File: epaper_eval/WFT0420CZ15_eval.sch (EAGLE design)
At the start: 15 parts, among them CN1 WFT0420CZ15_IF, CN2 WFT0420CZ15

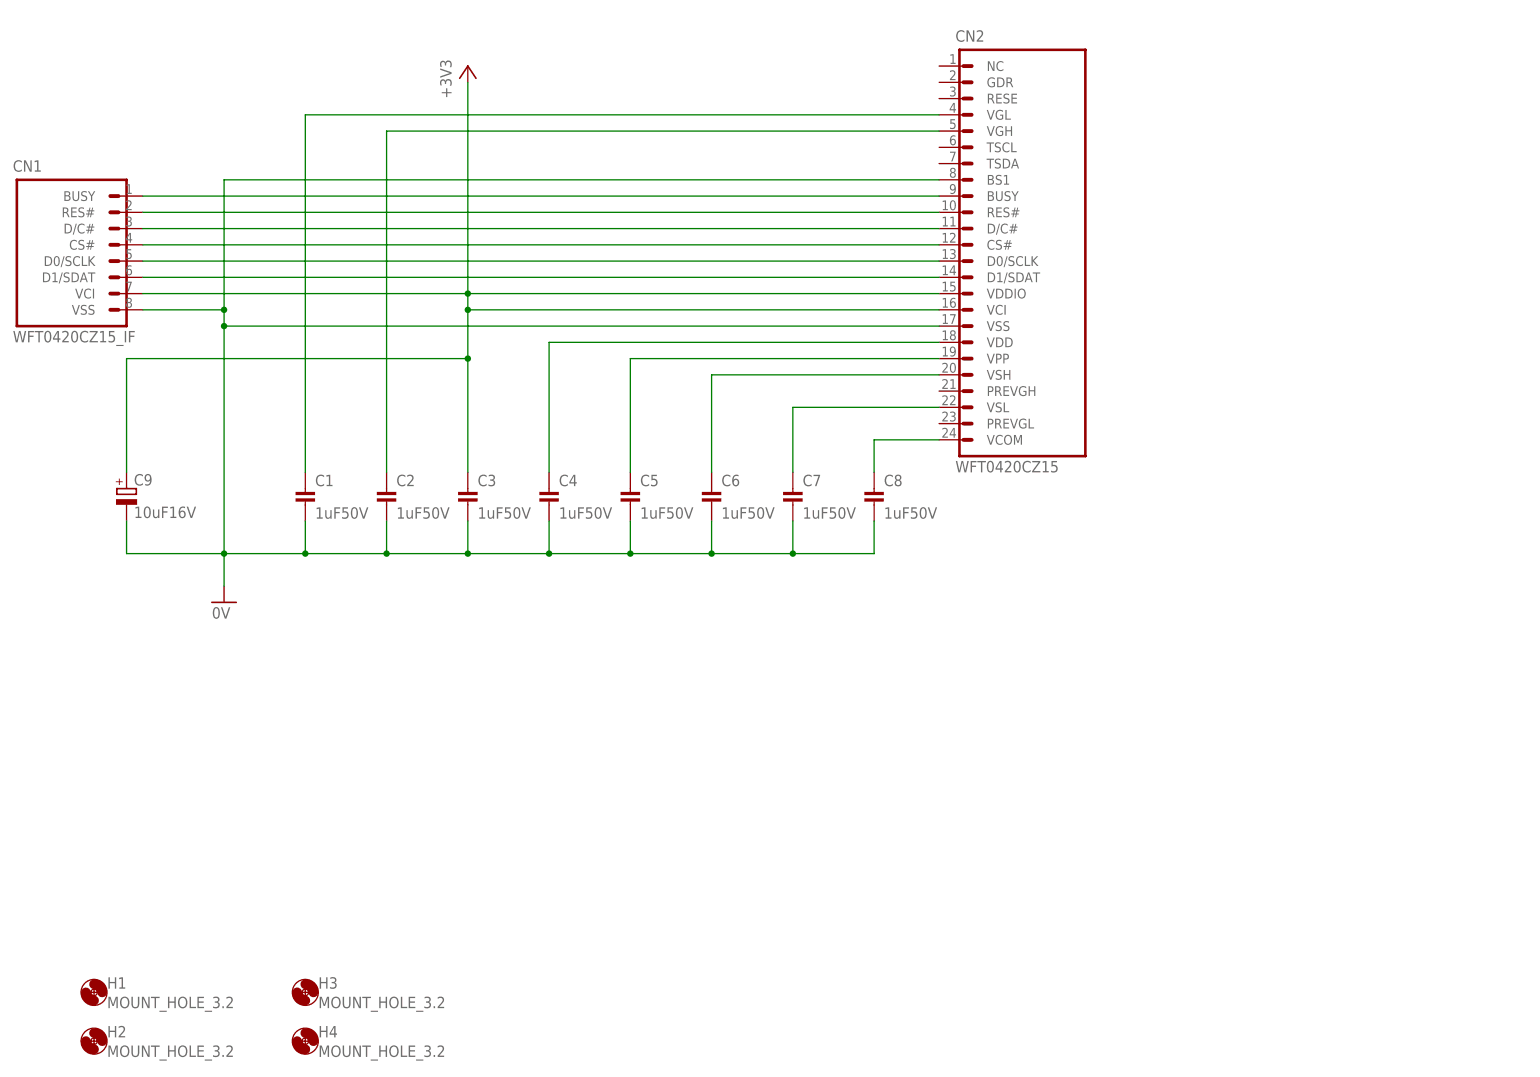
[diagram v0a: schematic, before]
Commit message: 部品を追加
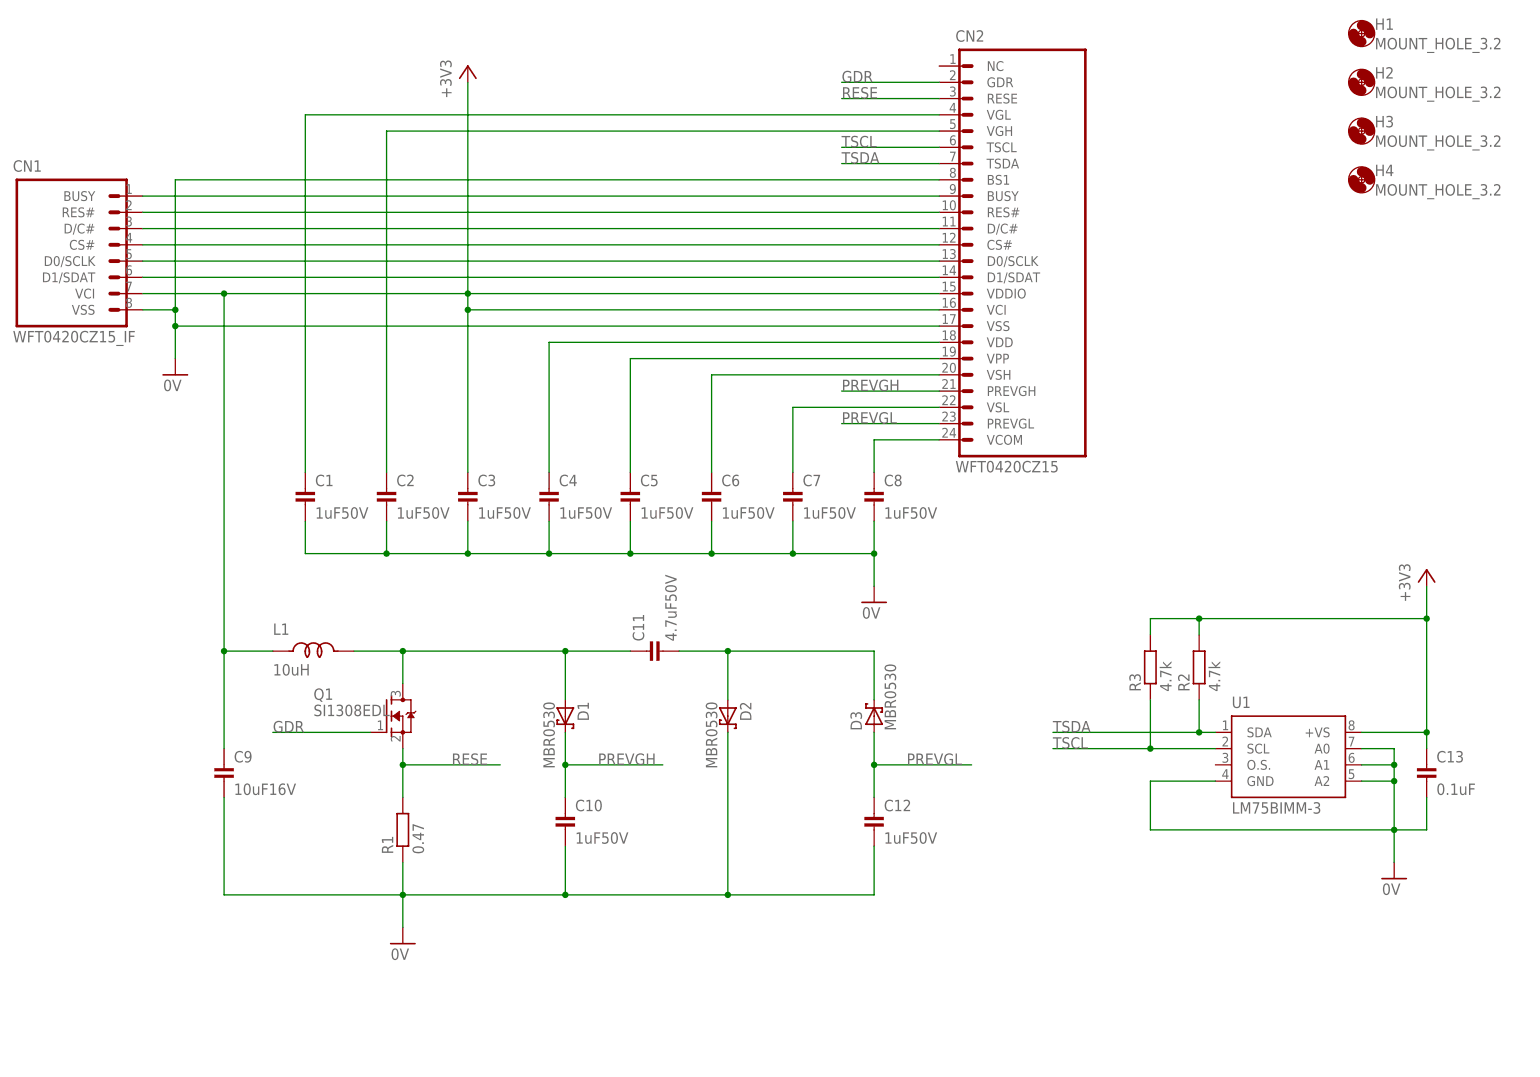
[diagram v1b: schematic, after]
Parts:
- added C10, C12: 1uF50V, Parts:CAP_0805
- added C11: 4.7uF50V, Parts:CAP_0805
- added C13: 0.1uF, Parts:CAP_0805
- added D1, D2, D3: MBR0530, Parts:MBR0530
- added L1: 10uH, Parts:NLCV25T
- added Q1: SI1308EDL, Parts:SI1308EDL
- added R1: 0.47, Parts:RESISTOR_0805
- added R2, R3: 4.7k, Parts:RESISTOR_0805
- added U1: LM75BIMM-3, Parts:LM75BIMM-3
- C9: device Parts:TPST106K016R0800 -> Parts:CAP_0805
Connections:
- new net GDR: CN2.GDR, Q1.G
- new net N$15: C11.2, D2.A, D3.C
- new net N$6: C11.1, D1.A, L1.2, Q1.D
- new net PREVGH: C10.1, CN2.PREVGH, D1.C
- new net PREVGL: C12.1, CN2.PREVGL, D3.A
- new net RESE: CN2.RESE, Q1.S, R1.2
- new net TSCL: CN2.TSCL, R3.1, U1.SCL
- new net TSDA: CN2.TSDA, R2.1, U1.SDA
- net +3V3: now also C13.1, C9.1, L1.1, R2.2, R3.2, U1.+VS; no longer C9.+
- net 0V: now also C10.2, C12.2, C13.2, C9.2, D2.C, R1.1, U1.A0, U1.A1, U1.A2, U1.GND; no longer C9.-
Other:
- moved on the sheet: H1, H2, H3, H4
